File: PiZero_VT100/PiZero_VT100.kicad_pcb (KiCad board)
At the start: 2 copper layers, 99.7 x 99.9 mm, 30 parts, among them J1 GPIO, J2 RS232, J3 Ext. Power max,. 9V DC/AC, J4 Mini-DIN-6, J5 to Testpins 22(DM) and TP23(D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, J6 USB_A, J7 Z80-MBC2 direct, J8 LCD Power, J9 On / Off, K1 G5V-2, Q1 BC547, U2 LM7805_TO220

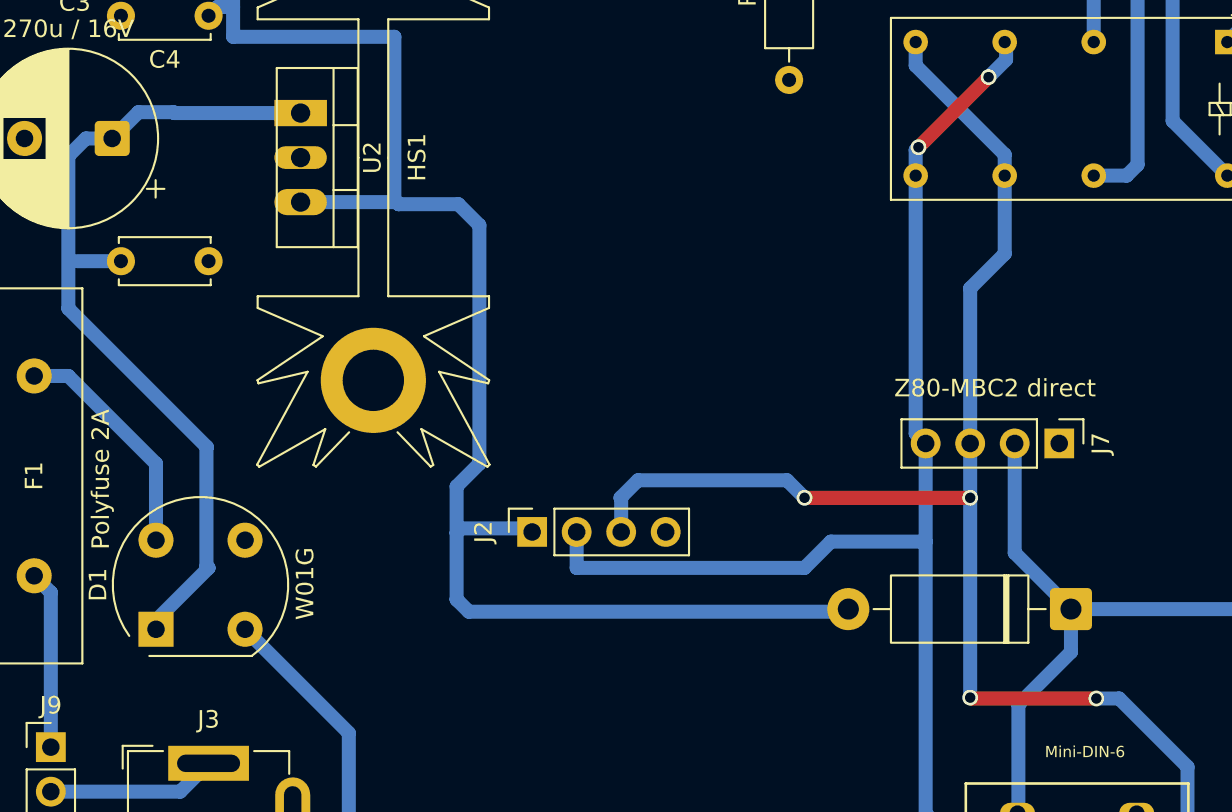
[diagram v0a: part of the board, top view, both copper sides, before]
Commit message: aktualisierung des Status
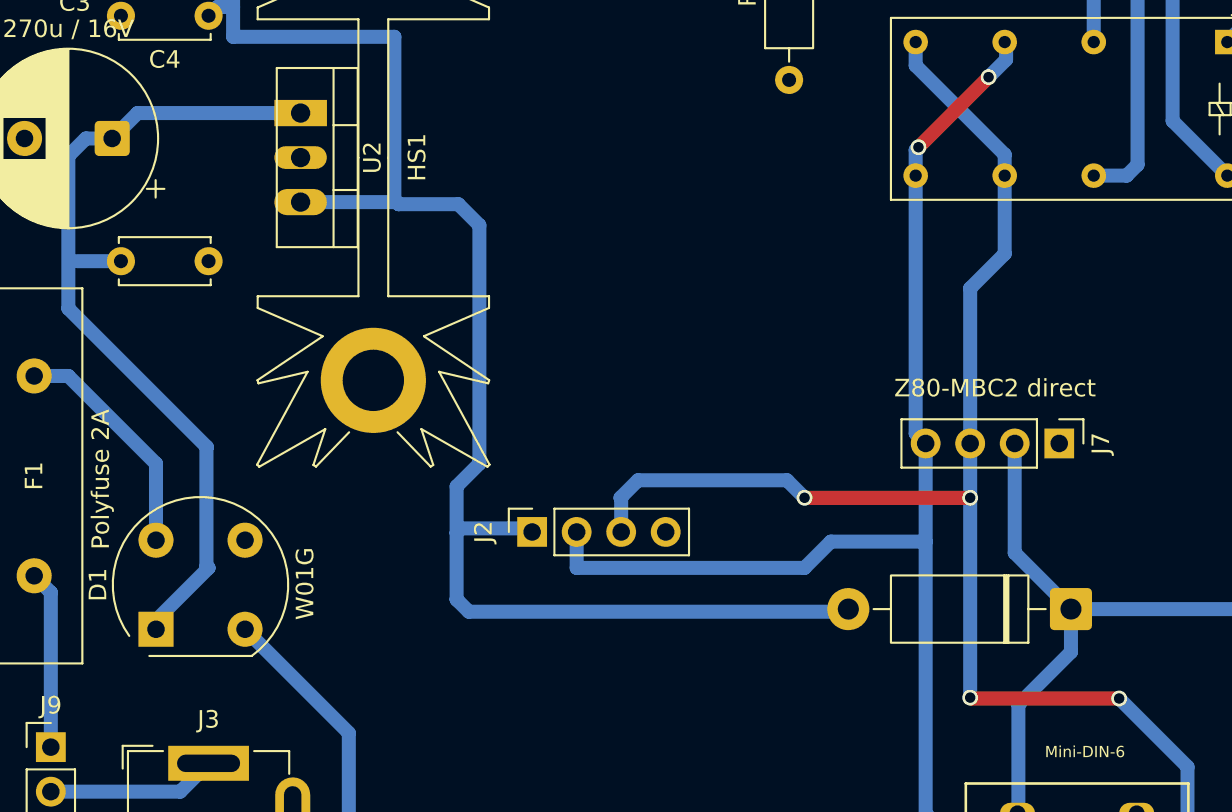
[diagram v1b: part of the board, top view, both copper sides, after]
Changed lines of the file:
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@@
-	)
-	(segment
-		(start 108.5 117.5)
-		(end 110.5 117.5)
-		(width 0.8)
-		(layer "B.Cu")
-		(net 35)
-	)
-	(segment
-		(start 110.55 117.55)
-		(end 117.75 117.55)
-		(width 0.8)
-		(layer "B.Cu")
-		(net 35)
-	)
-	(segment
-		(start 107 119)
-		(end 108.5 117.5)
-		(width 0.8)
-		(layer "B.Cu")
-		(net 35)
 	)
 	(segment
@@
 	(segment
 		(start 107 119)
+		(end 108.45 117.55)
+		(width 0.8)
+		(layer "B.Cu")
+		(net 35)
+	)
+	(segment
+		(start 107 119)
 		(end 105.5 119)
 		(width 0.8)
@@
 	)
 	(segment
-		(start 110.5 117.5)
-		(end 110.55 117.55)
-		(width 0.8)
-		(layer "B.Cu")
-		(net 35)
-	)
-	(segment
 		(start 112.379 136.621)
 		(end 112.379 143.379)
@@
 	)
 	(segment
+		(start 108.45 117.55)
+		(end 117.75 117.55)
+		(width 0.8)
+		(layer "B.Cu")
+		(net 35)
+	)
+	(segment
 		(start 112.379 143.379)
 		(end 112.5 143.5)
@@
 	)
 	(segment
-		(start 163.15 150.95)
+		(start 164.45 150.95)
 		(end 156 150.95)
 		(width 0.8)
@@
 	)
 	(via
-		(at 163.15 150.95)
+		(at 164.45 150.95)
 		(size 0.9)
 		(drill 0.6)
@@
 	)
 	(segment
+		(start 164.45 150.95)
+		(end 168.35 154.85)
+		(width 0.8)
+		(layer "B.Cu")
+		(net 49)
+	)
+	(segment
 		(start 137 138.5)
 		(end 136 139.5)
@@
 	)
 	(segment
-		(start 163.15 150.95)
-		(end 164.45 150.95)
-		(width 0.8)
-		(layer "B.Cu")
-		(net 49)
-	)
-	(segment
 		(start 145.5 138.5)
 		(end 137 138.5)
@@
 	)
 	(segment
+		(start 168.35 154.85)
+		(end 168.35 158.8)
+		(width 0.8)
+		(layer "B.Cu")
+		(net 49)
+	)
+	(segment
 		(start 146.5 139.5)
 		(end 145.5 138.5)
@@
 	)
 	(segment
-		(start 164.45 150.95)
-		(end 168.35 154.85)
-		(width 0.8)
-		(layer "B.Cu")
-		(net 49)
-	)
-	(segment
-		(start 168.35 154.85)
-		(end 168.35 158.8)
-		(width 0.8)
-		(layer "B.Cu")
-		(net 49)
-	)
-	(segment
 		(start 152.84 114.84)
 		(end 157.92 119.92)
@@
 	)
 	(segment
+		(start 155.95 136.4)
+		(end 155.95 139.5)
+		(width 0.8)
+		(layer "B.Cu")
+		(net 49)
+	)
+	(segment
+		(start 152.84 113.5)
+		(end 152.84 114.84)
+		(width 0.8)
+		(layer "B.Cu")
+		(net 49)
+	)
+	(segment
+		(start 167.15 160)
+		(end 165.45 160)
+		(width 0.8)
+		(layer "B.Cu")
+		(net 49)
+	)
+	(segment
 		(start 168.35 158.8)
 		(end 167.15 160)
 		(width 0.8)
 		(layer "B.Cu")
-		(net 49)
-	)
-	(segment
-		(start 155.95 136.4)
-		(end 155.95 139.5)
-		(width 0.8)
-		(layer "B.Cu")
-		(net 49)
-	)
-	(segment
-		(start 152.84 113.5)
-		(end 152.84 114.84)
-		(width 0.8)
-		(layer "B.Cu")
-		(net 49)
-	)
-	(segment
-		(start 167.15 160)
-		(end 165.45 160)
-		(width 0.8)
-		(layer "B.Cu")
